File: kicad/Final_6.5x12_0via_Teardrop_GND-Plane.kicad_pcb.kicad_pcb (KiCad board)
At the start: 2 copper layers, 33.6 x 17.7 mm, 18 parts, among them J3 FDTI, SW1 SW_Push, U1 ATmega328P-A

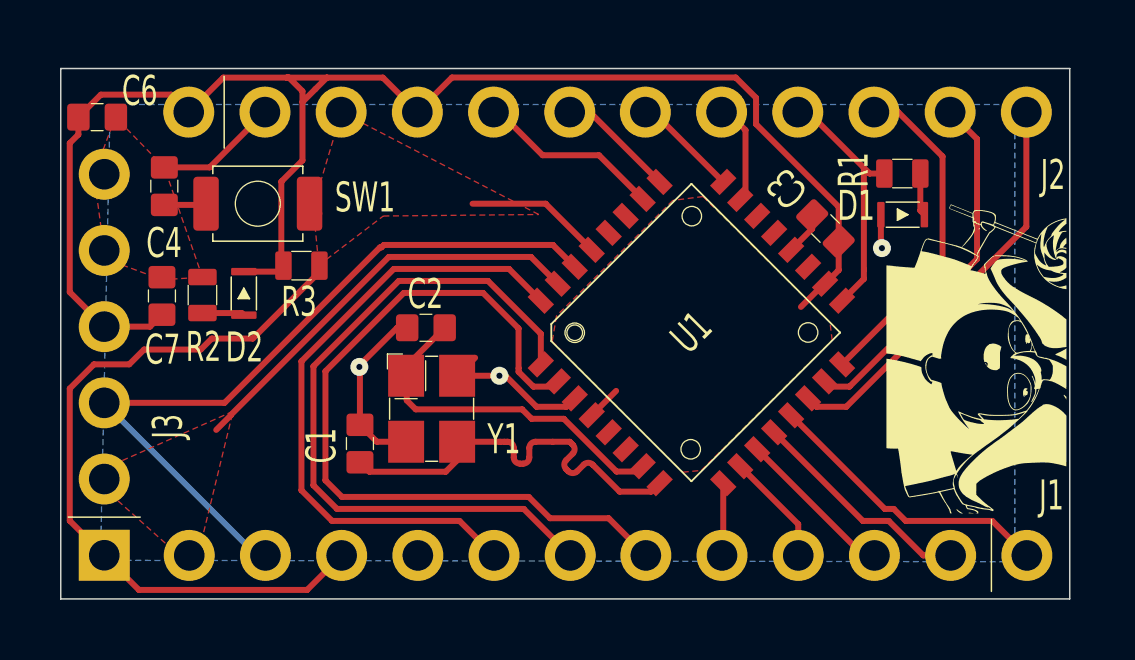
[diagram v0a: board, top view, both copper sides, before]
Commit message: a
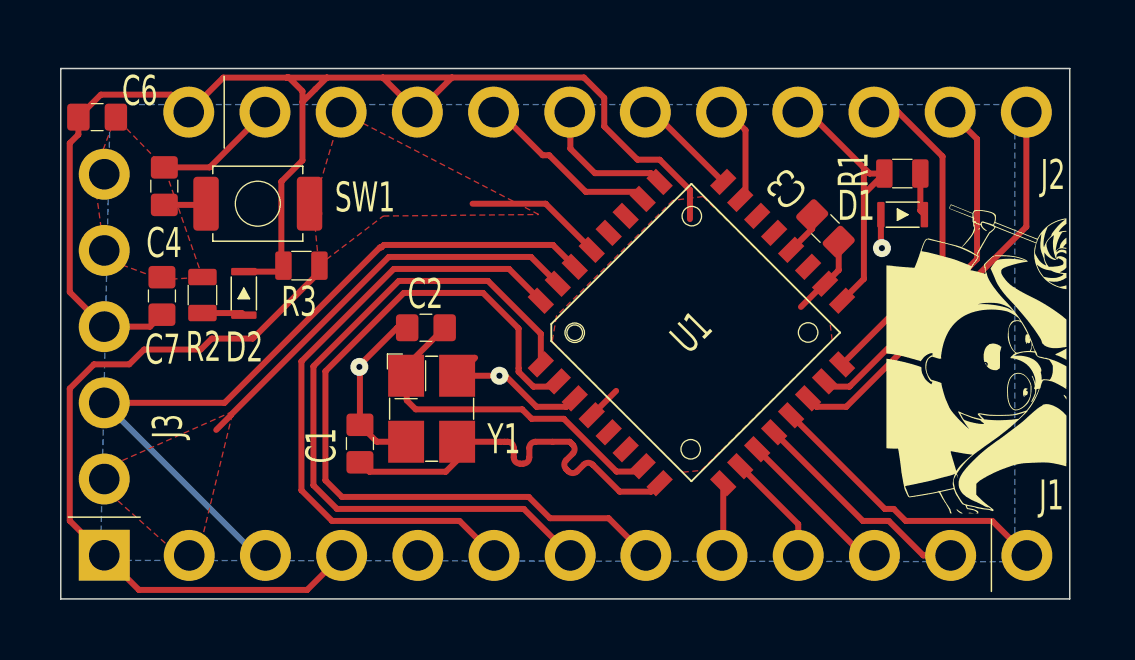
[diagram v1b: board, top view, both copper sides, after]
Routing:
- net RAW: track 53.7 -> 50.7 mm
- net SCK: track 8.58 -> 9.55 mm
- net A2: track 4.07 -> 4.98 mm
